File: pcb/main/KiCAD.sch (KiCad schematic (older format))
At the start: 368 parts, among them Q1 2N7002, SW1 CherryMX, SW10 CherryMX, SW11 CherryMX, SW12 CherryMX, SW13 CherryMX, SW14 CherryMX, SW15 CherryMX, SW16 CherryMX, SW17 CherryMX, SW18 CherryMX, SW19 CherryMX, SW2 CherryMX, SW20 CherryMX, SW21 CherryMX, SW22 CherryMX, SW23 CherryMX, SW24 CherryMX, SW25 CherryMX, SW26 CherryMX, SW27 CherryMX, SW28 CherryMX, SW29 CherryMX, SW3 CherryMX, SW30 CherryMX, SW31 CherryMX, SW32 CherryMX, SW33 CherryMX, SW34 CherryMX, SW35 CherryMX, SW36 CherryMX, SW37 CherryMX, SW38 CherryMX, SW39 CherryMX, SW4 CherryMX, SW40 CherryMX, SW41 CherryMX, SW42 CherryMX, SW43 CherryMX, SW44 CherryMX, SW45 CherryMX, SW46 CherryMX, SW47 CherryMX, SW48 CherryMX, SW49 CherryMX, SW5 CherryMX, SW50 CherryMX, SW51 CherryMX, SW52 CherryMX, SW53 CherryMX, SW54 CherryMX, SW55 CherryMX, SW56 CherryMX, SW57 CherryMX, SW58 CherryMX, SW59 CherryMX, SW6 CherryMX, SW60 CherryMX, SW61 CherryMX, SW62 CherryMX, SW63 CherryMX, SW64 CherryMX, SW65 CherryMX, SW66 CherryMX, SW67 CherryMX, SW68 CherryMX, SW69 CherryMX, SW7 CherryMX, SW70 CherryMX, SW71 CherryMX, SW72 CherryMX, SW73 CherryMX, SW74 CherryMX, SW75 CherryMX, SW76 CherryMX, SW77 CherryMX, SW78 CherryMX, SW79 CherryMX, SW8 CherryMX, SW80 CherryMX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

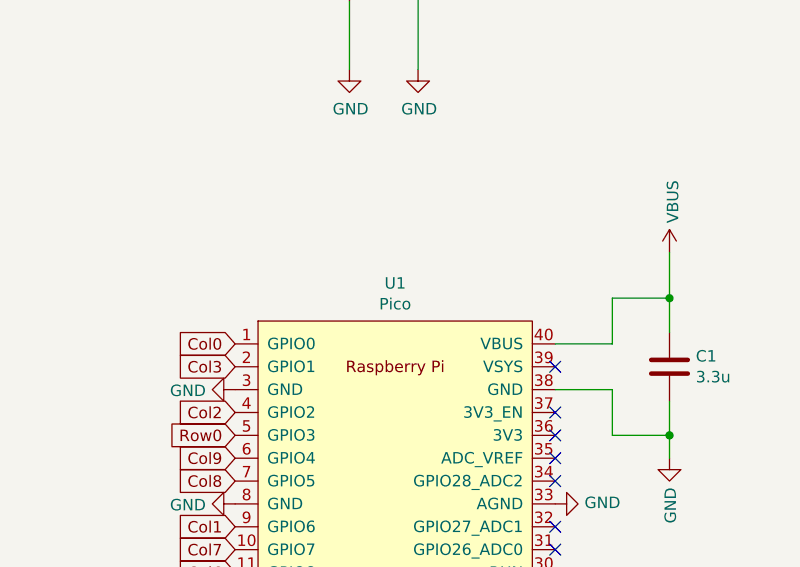
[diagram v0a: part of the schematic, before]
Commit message: Add files via upload
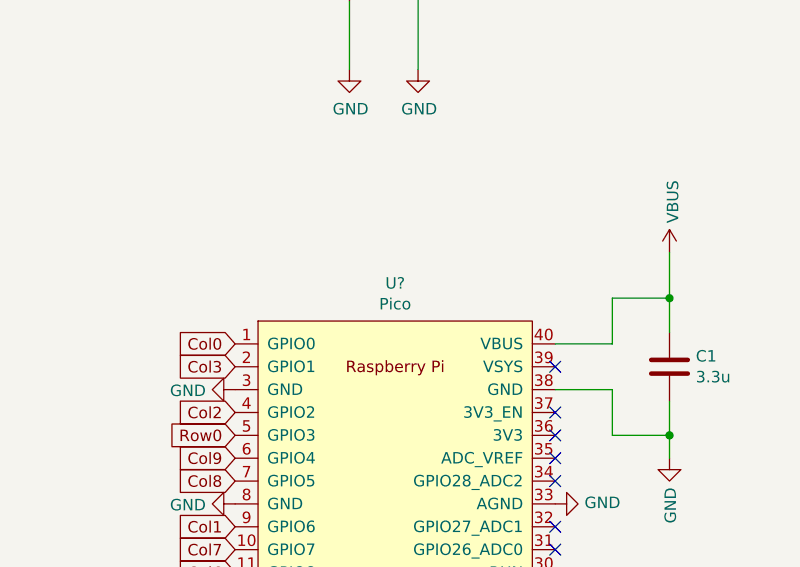
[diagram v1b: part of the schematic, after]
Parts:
- removed U1: Pico, RPi_Pico:RPi_Pico_SMD_TH, symbol KiCAD-rescue:Pico-RaspberryPi_Pico
- added U?: Pico, RPi_Pico:RPi_Pico_SMD_TH, symbol RaspberryPi_Pico:Pico
- C1: footprint (none) -> Capacitor_SMD:C_0603_1608Metric
- R89: footprint (none) -> Resistor_SMD:R_0603_1608Metric
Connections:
- net Col0: now also U?.1 (GPIO0)
- net Col1: now also U?.9 (GPIO6)
- net Col2: now also U?.4 (GPIO2)
- net Col3: now also U?.2 (GPIO1)
- net Col4: now also U?.14 (GPIO10)
- net Col5: now also U?.12 (GPIO9)
- net Col6: now also U?.11 (GPIO8)
- net Col7: now also U?.10 (GPIO7)
- net Col8: now also U?.7 (GPIO5)
- net Col9: now also U?.6 (GPIO4)
- net GND: now also U?.13 (GND), U?.18 (GND), U?.23 (GND), U?.28 (GND), U?.3 (GND), U?.33 (AGND), U?.38 (GND), U?.8 (GND)
- net PWM: now also U?.29 (GPIO22)
- net Row0: now also U?.5 (GPIO3)
- net Row1: now also U?.15 (GPIO11)
- net Row2: now also U?.17 (GPIO13)
- net Row3: now also U?.16 (GPIO12)
- net Row4: now also U?.19 (GPIO14)
- net Row5: now also U?.20 (GPIO15)
- net Row6: now also U?.27 (GPIO21)
- net Row7: now also U?.26 (GPIO20)
- net Row8: now also U?.25 (GPIO19)
- net Row9: now also U?.24 (GPIO18)
- net VBUS: now also U?.40 (VBUS)
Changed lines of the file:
@@
-$EndComp
-$Comp
-L KiCAD-rescue:Pico-RaspberryPi_Pico U1
-U 1 1 63A3E8CA
-P 2250 7850
-F 0 "U1" H 2250 9065 50  0000 C CNN
-F 1 "Pico" H 2250 8974 50  0000 C CNN
-F 2 "RPi_Pico:RPi_Pico_SMD_TH" V 2250 7850 50  0001 C CNN
-F 3 "" H 2250 7850 50  0001 C CNN
-	1    2250 7850
-	1    0    0    -1
 $EndComp
 $Comp
@@
 F 0 "C1" H 3565 7046 50  0000 L CNN
 F 1 "3.3u" H 3565 6955 50  0000 L CNN
-F 2 "" H 3488 6850 50  0001 C CNN
+F 2 "Capacitor_SMD:C_0603_1608Metric" H 3488 6850 50  0001 C CNN
 F 3 "~" H 3450 7000 50  0001 C CNN
 	1    3450 7000
@@
 F 0 "R89" H 2120 5296 50  0000 L CNN
 F 1 "10k" H 2120 5205 50  0000 L CNN
-F 2 "" V 1980 5250 50  0001 C CNN
+F 2 "Resistor_SMD:R_0603_1608Metric" V 1980 5250 50  0001 C CNN
 F 3 "~" H 2050 5250 50  0001 C CNN
 	1    2050 5250
@@
 Wire Wire Line
 	3450 7300 3450 7400
+$Comp
+L RaspberryPi_Pico:Pico U?
+U 1 1 61447957
+P 2250 7850
+F 0 "U?" H 2250 9065 50  0000 C CNN
+F 1 "Pico" H 2250 8974 50  0000 C CNN
+F 2 "RPi_Pico:RPi_Pico_SMD_TH" V 2250 7850 50  0001 C CNN
+F 3 "" H 2250 7850 50  0001 C CNN
+	1    2250 7850
+	1    0    0    -1
+$EndComp
 $EndSCHEMATC

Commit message: 復元した
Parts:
- removed U?: Pico, RPi_Pico:RPi_Pico_SMD_TH, symbol RaspberryPi_Pico:Pico
- added U?: Pico, RPi_Pico:RPi_Pico_SMD_TH, symbol RaspberryPi_Pico:Pico
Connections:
- net Col0: now also U?.1 (GPIO0)
- net Col1: now also U?.9 (GPIO6)
- net Col2: now also U?.4 (GPIO2)
- net Col3: now also U?.2 (GPIO1)
- net Col4: now also U?.14 (GPIO10)
- net Col5: now also U?.12 (GPIO9)
- net Col6: now also U?.11 (GPIO8)
- net Col7: now also U?.10 (GPIO7)
- net Col8: now also U?.7 (GPIO5)
- net Col9: now also U?.6 (GPIO4)
- net GND: now also U?.13 (GND), U?.18 (GND), U?.23 (GND), U?.28 (GND), U?.3 (GND), U?.33 (AGND), U?.38 (GND), U?.8 (GND)
- net PWM: now also U?.29 (GPIO22)
- net Row0: now also U?.5 (GPIO3)
- net Row1: now also U?.15 (GPIO11)
- net Row2: now also U?.17 (GPIO13)
- net Row3: now also U?.16 (GPIO12)
- net Row4: now also U?.19 (GPIO14)
- net Row5: now also U?.20 (GPIO15)
- net Row6: now also U?.27 (GPIO21)
- net Row7: now also U?.26 (GPIO20)
- net Row8: now also U?.25 (GPIO19)
- net Row9: now also U?.24 (GPIO18)
- net VBUS: now also U?.40 (VBUS)
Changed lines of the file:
@@
 $Comp
 L RaspberryPi_Pico:Pico U?
-U 1 1 61447957
+U 1 1 6143F7AA
 P 2250 7850
 F 0 "U?" H 2250 9065 50  0000 C CNN
